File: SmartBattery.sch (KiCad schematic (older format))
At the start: 22 parts, among them J12 Conn_01x10_Male, J13 Conn_01x03_Male, Q22 AO3401A, U14 HT7533-1

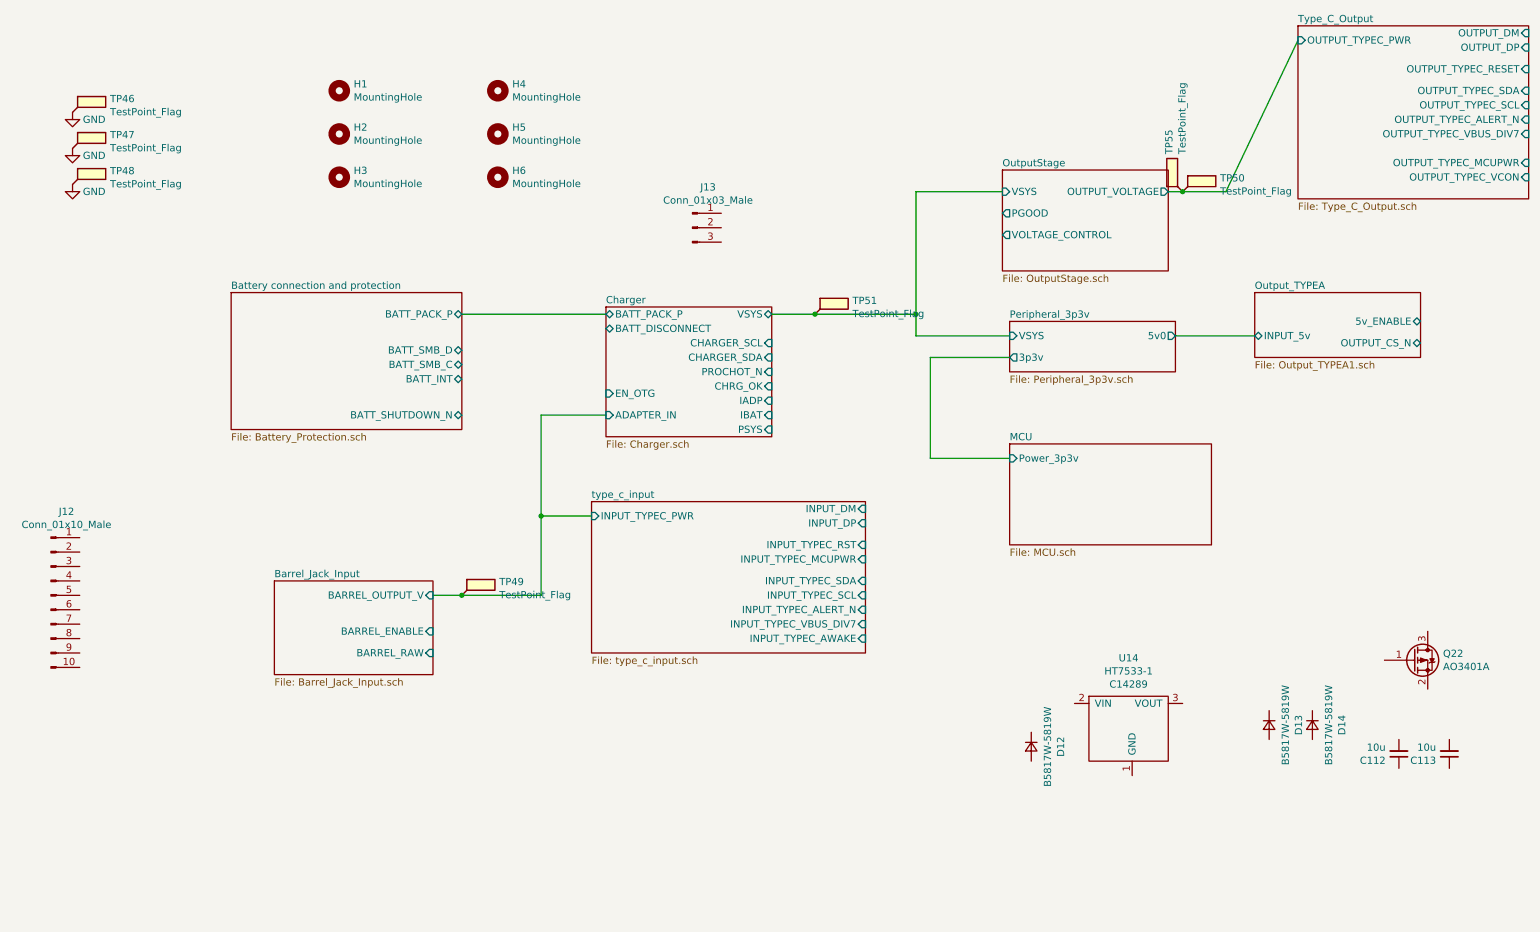
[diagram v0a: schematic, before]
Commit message: Much layout wow.
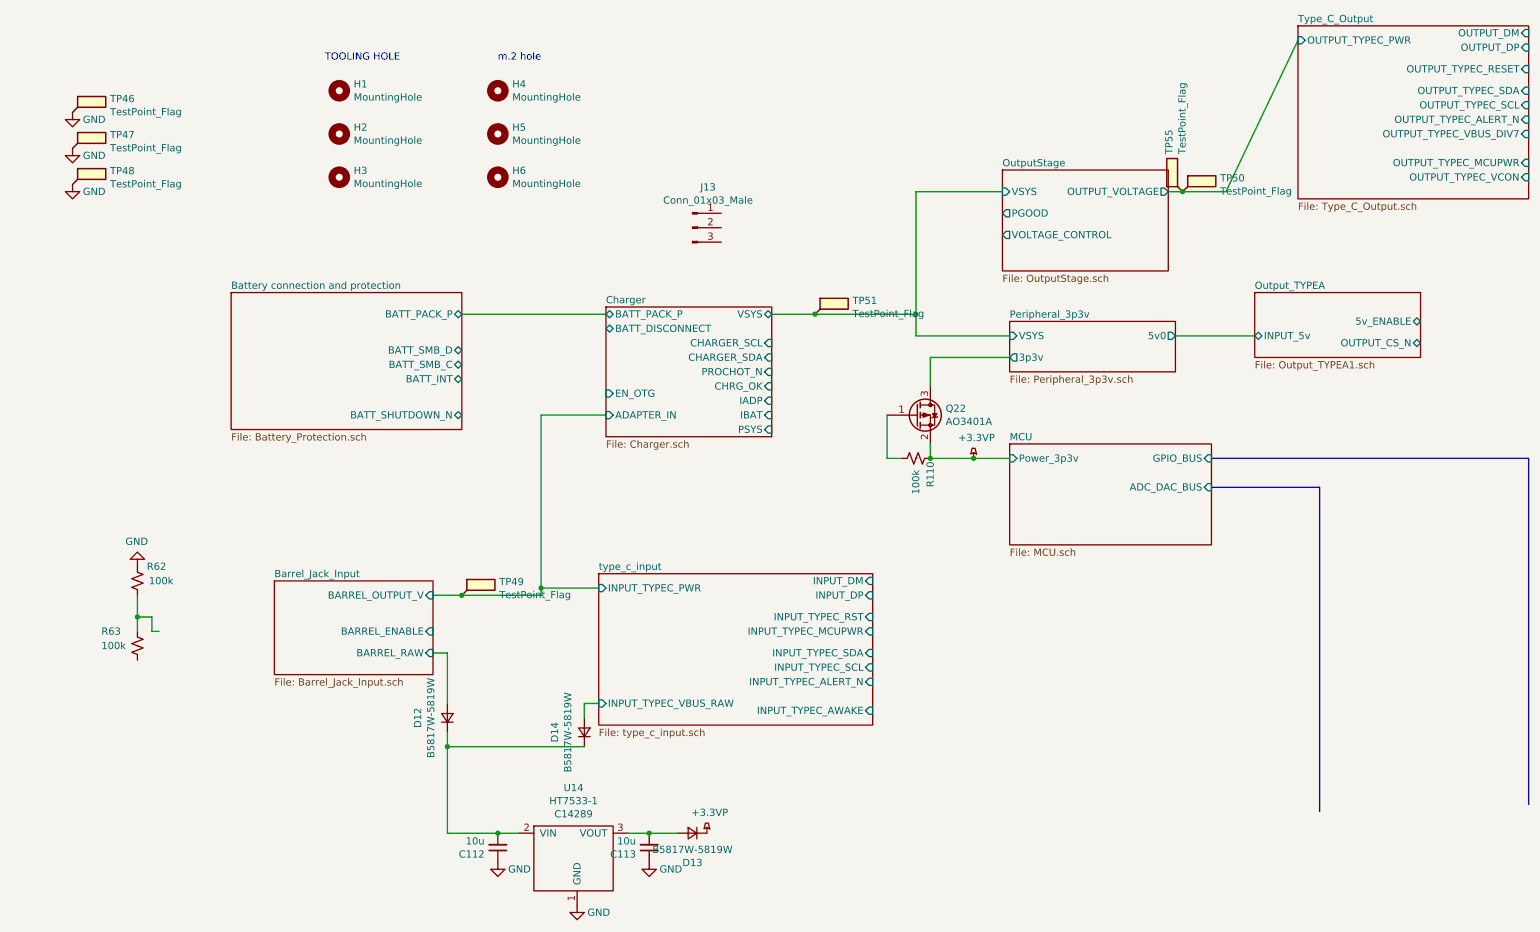
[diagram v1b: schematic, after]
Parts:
- removed J12: Conn_01x10_Male, Connector_PinHeader_1.27mm:PinHeader_2x05_P1.27mm_Vertical_SMD, symbol Connector:Conn_01x10_Male
- added R110, R62, R63: 100k, lc_lib:0402_R, symbol Device:R_Small_US
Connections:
- net Barrel_Jack_Input/BARREL_RAW: now also D12.2 (A)
- net GND: now also C112.1, C113.1, U14.1 (GND), R62.2
- net at U14.2 (VIN): now also C112.2, D12.1 (K), D14.1 (K)
- net at U14.3 (VOUT): now also C113.2, D13.2 (A)
- net +3.3VP: now reaches D13.1 (K)
- net +3.3VP: now also Q22.2 (S), R110.2
- net type_c_input/INPUT_TYPEC_VBUS_RAW: now reaches D14.2 (A)
- net at Q22.1 (G): now also R110.1
- net Peripheral_3p3v/3p3v: now reaches Q22.3 (D)
- new net: R62.1, R63.1
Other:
- note added: "TOOLING HOLE\n"
- note added: "m.2 hole\n"
- moved on the sheet: C112, C113, D12, D13, D14, Q22, U14
